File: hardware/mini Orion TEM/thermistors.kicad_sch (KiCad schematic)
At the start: 26 parts, among them U201 SN74LV4051A-Q1

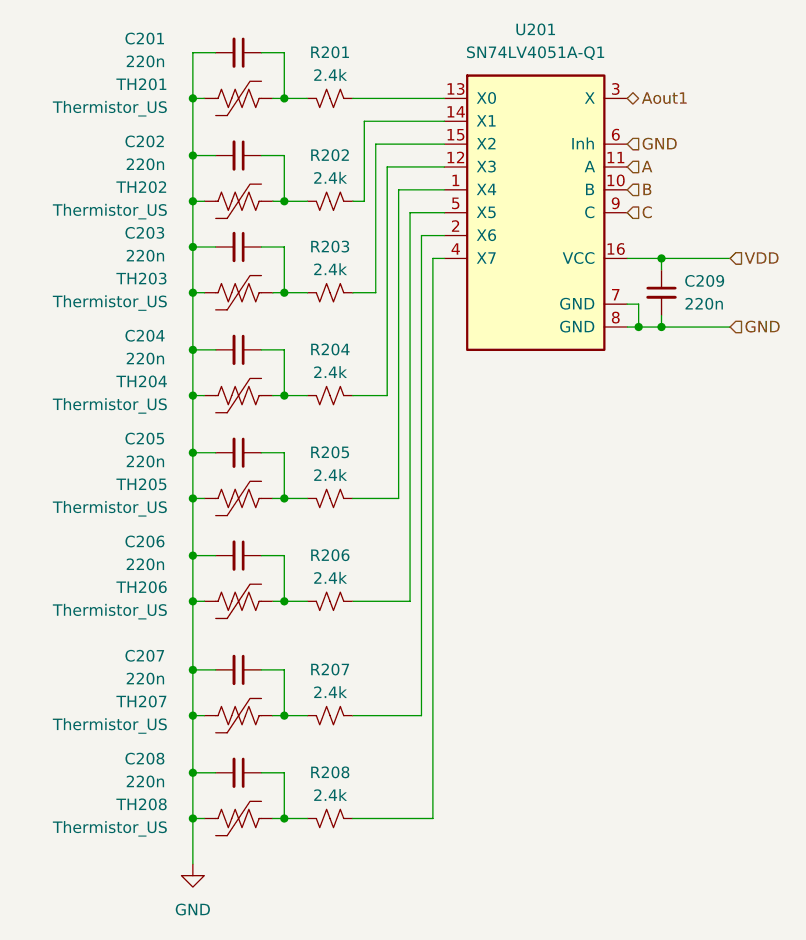
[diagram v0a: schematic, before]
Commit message: NOTHING MATCHES CAD!!!!!!!!!
YIPPERS!!
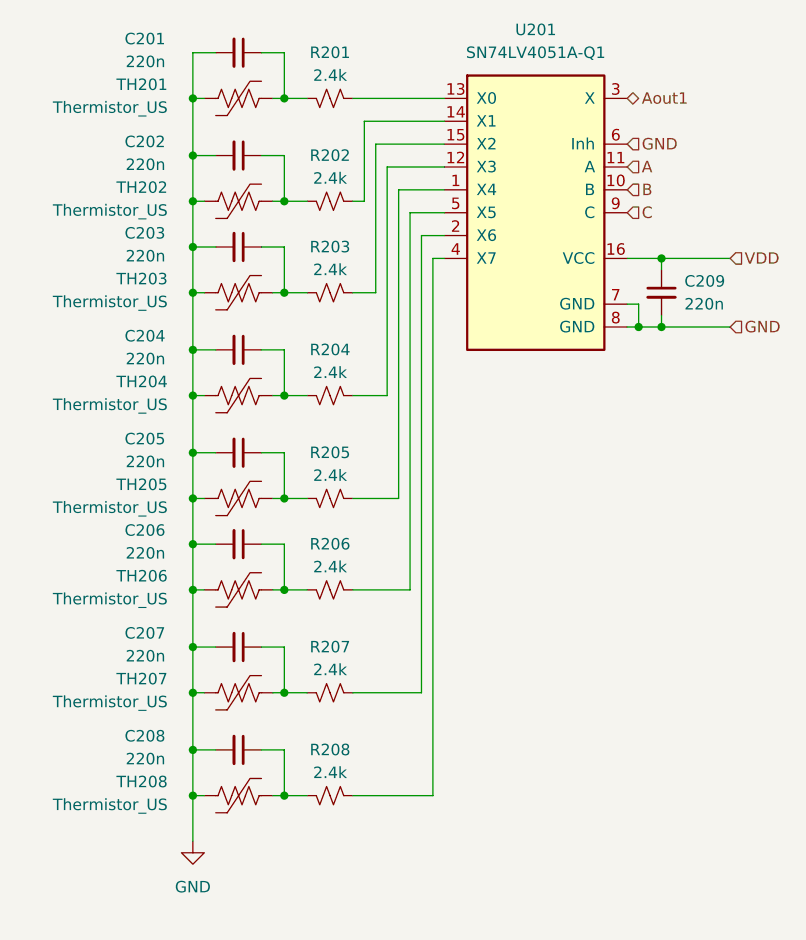
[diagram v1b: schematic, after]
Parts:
- TH201, TH202, TH203, TH204, TH205, TH206, TH207, TH208: footprint Resistor_SMD:R_1206_3216Metric -> zzLocalLibraries-Footprints:FPC thermistor strip 2x2mm
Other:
- moved on the sheet: C206, C207, C208, R206, R207, R208
